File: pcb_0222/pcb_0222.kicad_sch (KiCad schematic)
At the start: 94 parts, among them J1 S2P-VH, J2 SM02B-PASS-TBT, J3 SM02B-PASS-TBT, J4 SM08B-PASS-TBT, J5 TC-2030-IDC, J6 SM08B-PASS-TBT, J7 HEADER_MALE_THT_0.1"_4x1, J8 HEADER_MALE_THT_0.1"_2x1, J9 HEADER_MALE_THT_0.1"_4x1, K1 EE2-3NUH, Q1 BSP170PH6327XTSA1, Q2 BC817-16, U1 LMR54406DBVR, U2 STM32C011F6P6

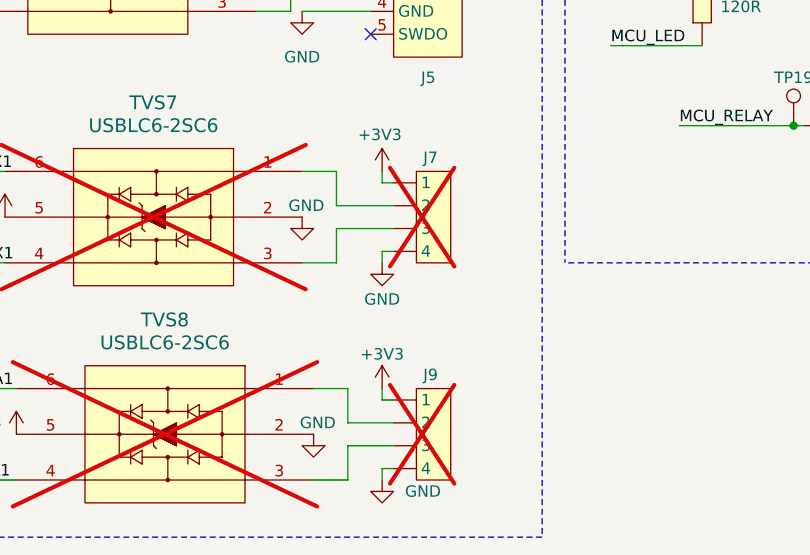
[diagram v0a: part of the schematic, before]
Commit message: Layout Review Pending + Preliminary Manufacturer Package Generated
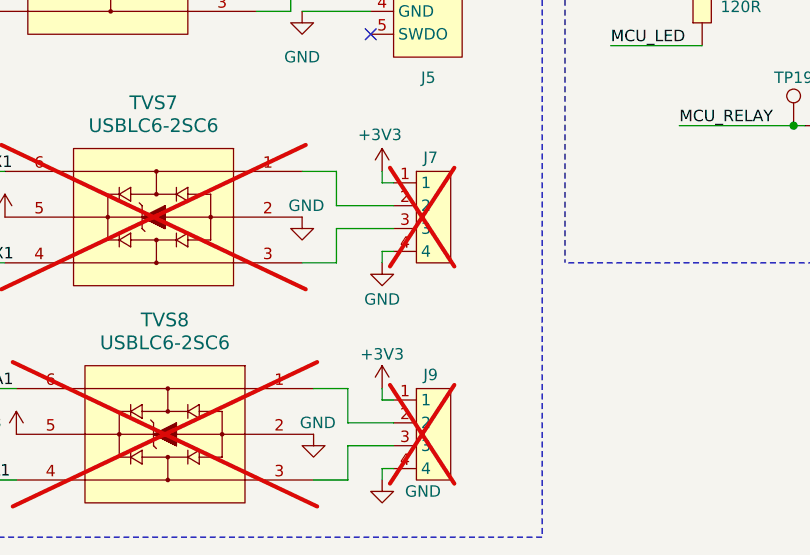
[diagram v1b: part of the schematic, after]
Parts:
- J7, J9: DIGIKEY_PN_CT (none) -> 732-5317-ND; MANUFACTURER (none) -> Würth Elektronik
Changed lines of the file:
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@@
 			)
 		)
+		(property "MANUFACTURER" "Würth Elektronik"
+			(at 152.4 185.42 0)
+			(hide yes)
+			(show_name no)
+			(do_not_autoplace no)
+			(effects
+				(font
+					(size 1.27 1.27)
+				)
+			)
+		)
+		(property "DIGIKEY_PN_CT" "732-5317-ND"
+			(at 152.4 185.42 0)
+			(hide yes)
+			(show_name no)
+			(do_not_autoplace no)
+			(effects
+				(font
+					(size 1.27 1.27)
+				)
+			)
+		)
 		(pin "4"
 		)
@@
 			(at 152.4 161.29 0)
 			(hide yes)
+			(show_name no)
+			(do_not_autoplace no)
+			(effects
+				(font
+					(size 1.27 1.27)
+				)
+			)
+		)
+		(property "MANUFACTURER" "Würth Elektronik"
+			(at 152.4 161.29 0)
+			(hide yes)
+			(show_name no)
+			(do_not_autoplace no)
+			(effects
+				(font
+					(size 1.27 1.27)
+				)
+			)
+		)
+		(property "DIGIKEY_PN_CT" "732-5317-ND"
+			(at 152.4 161.29 0)
+			(hide yes)
